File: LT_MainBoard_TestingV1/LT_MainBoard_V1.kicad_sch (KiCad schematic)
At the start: 24 parts, among them CN1 NUCLEO-L432KC, J1 Molar Nanofit Connectors, U1 ISO1050DUB, U2 MCP2515-I/SO, U3 317990687, U4 LM7809_TO220, U5 LM7805_TO220, U6 LM3480-3.3

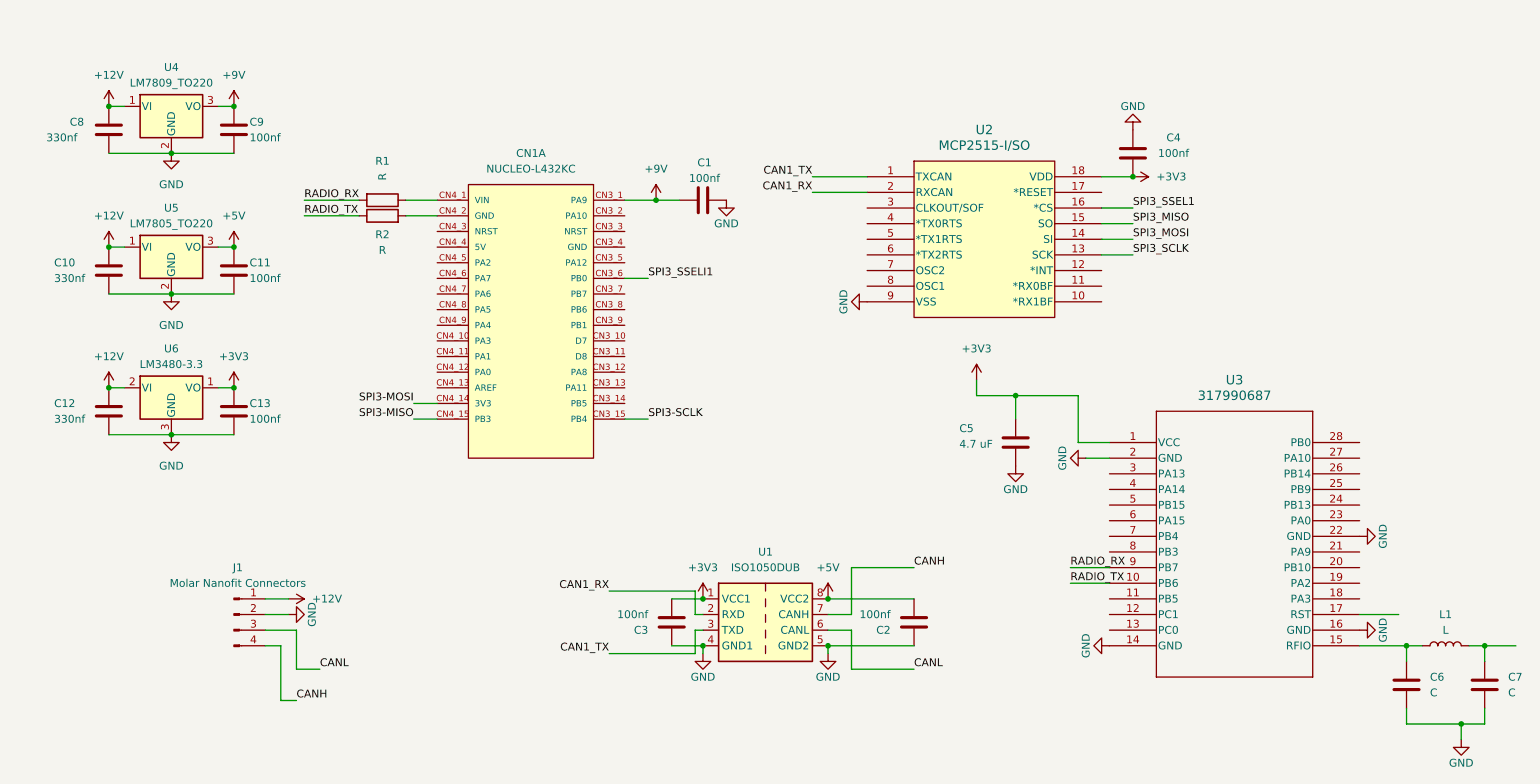
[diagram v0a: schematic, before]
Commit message: Adapter V1
Made adapter board, modified lt mainboard
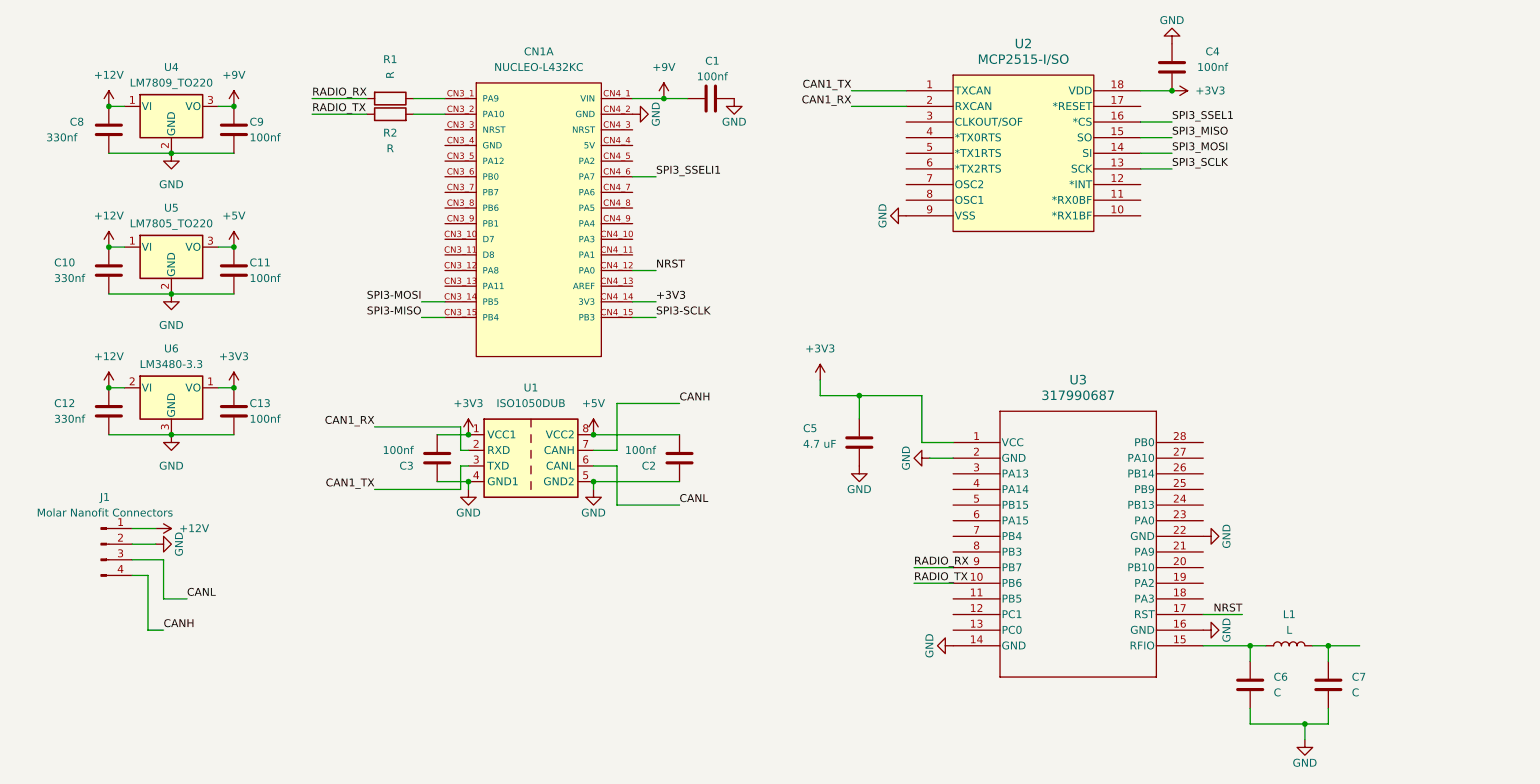
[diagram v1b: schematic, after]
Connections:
- net +3V3: now also CN1.CN4_14 (3V3)
- net +9V: now also CN1.CN4_1 (VIN); no longer CN1.CN3_1 (PA9)
- net GND: now also CN1.CN4_2 (GND)
- net SPI3-MISO: now also CN1.CN3_15 (PB4); no longer CN1.CN4_15 (PB3)
- net SPI3-MOSI: now also CN1.CN3_14 (PB5); no longer CN1.CN4_14 (3V3)
- net SPI3-SCLK: now also CN1.CN4_15 (PB3); no longer CN1.CN3_15 (PB4)
- net SPI3_SSELI1: now also CN1.CN4_6 (PA7); no longer CN1.CN3_6 (PB0)
- net at CN1.CN3_2 (PA10): now also R2.2
- net at R1.1: now also CN1.CN3_1 (PA9); no longer CN1.CN4_1 (VIN)
- net NRST: now reaches CN1.CN4_12 (PA0)
- net NRST: now also U3.17 (RST)
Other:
- title: (none) -> Live Telemetry Testing Board
- moved on the sheet: C1, C2, C3, C4, C5, C6, C7, CN1A, J1, L1, R1, R2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
